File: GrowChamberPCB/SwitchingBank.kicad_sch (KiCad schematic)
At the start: 14 parts, among them J11 TP, J17 TP, J18 TP, J19 TP, J20 TP, J21 TP, Q17 NPN, Q18 MOSFET, Q8 BRT30N70P3, Q9 NPN

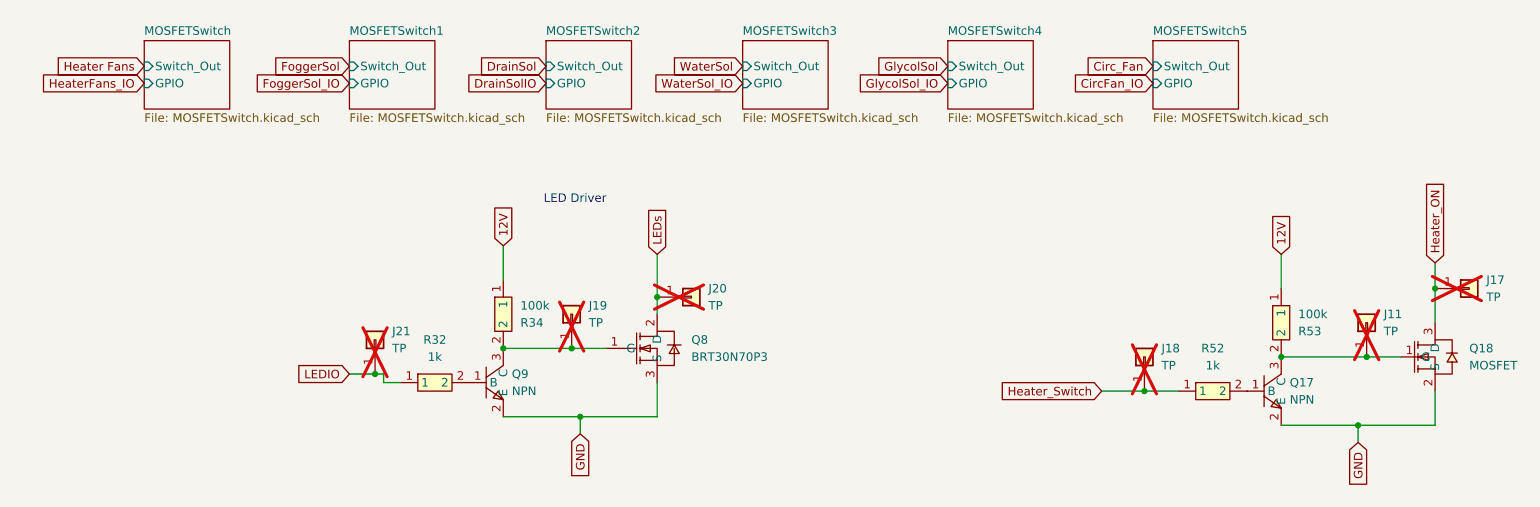
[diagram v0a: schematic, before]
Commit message: finished routing
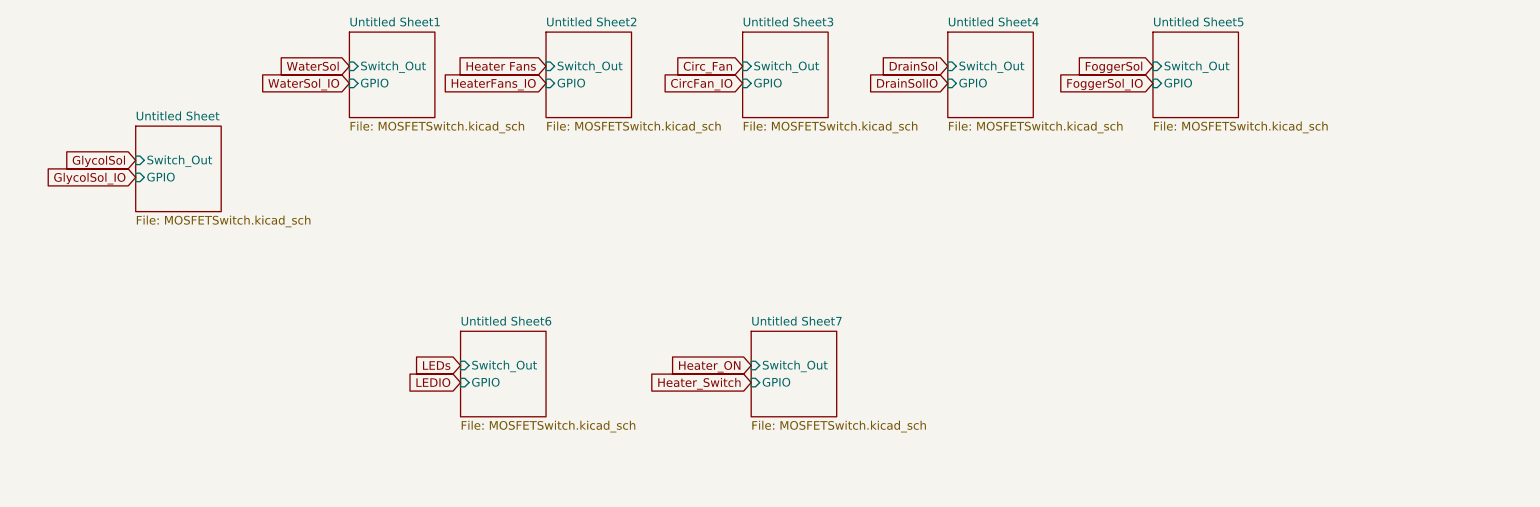
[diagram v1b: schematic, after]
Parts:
- removed J11, J17, J18, J19, J20, J21: TP, TestPoint:TestPoint_Pad_D2.0mm, symbol Connector_Generic:Conn_01x01
- removed Q17, Q9: NPN, easyeda2kicad:SOT-23-3_L3.0-W1.7-P0.95-LS2.9-BR, symbol easyeda2kicad:2N22221P-TD
- removed Q18: MOSFET, easyeda2kicad:SOT-23-3_L2.9-W1.3-P1.90-LS2.4-BR, symbol easyeda2kicad:AO3400A_C347475
- removed Q8: BRT30N70P3, easyeda2kicad:TO-252-2_L6.6-W6.1-P4.60-LS10.0-BR-CW, symbol easyeda2kicad:BRT30N70P3
- removed R32, R52: 1k, easyeda2kicad:R0603, symbol easyeda2kicad:FRC0603J102TS
- removed R34, R53: 100k, easyeda2kicad:R0603, symbol easyeda2kicad:FRC0603F1004TS
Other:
- removed sheet MOSFETSwitch
- removed sheet MOSFETSwitch1
- removed sheet MOSFETSwitch2
- removed sheet MOSFETSwitch3
- removed sheet MOSFETSwitch4
- removed sheet MOSFETSwitch5
- added sheet Untitled Sheet (MOSFETSwitch.kicad_sch)
- added sheet Untitled Sheet1 (MOSFETSwitch.kicad_sch)
- added sheet Untitled Sheet2 (MOSFETSwitch.kicad_sch)
- added sheet Untitled Sheet3 (MOSFETSwitch.kicad_sch)
- added sheet Untitled Sheet4 (MOSFETSwitch.kicad_sch)
- added sheet Untitled Sheet5 (MOSFETSwitch.kicad_sch)
- added sheet Untitled Sheet6 (MOSFETSwitch.kicad_sch)
- added sheet Untitled Sheet7 (MOSFETSwitch.kicad_sch)
- note removed: "LED Driver"
